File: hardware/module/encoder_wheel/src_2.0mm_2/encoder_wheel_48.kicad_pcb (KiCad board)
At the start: 2 copper layers, 74 x 74 mm, 2 parts

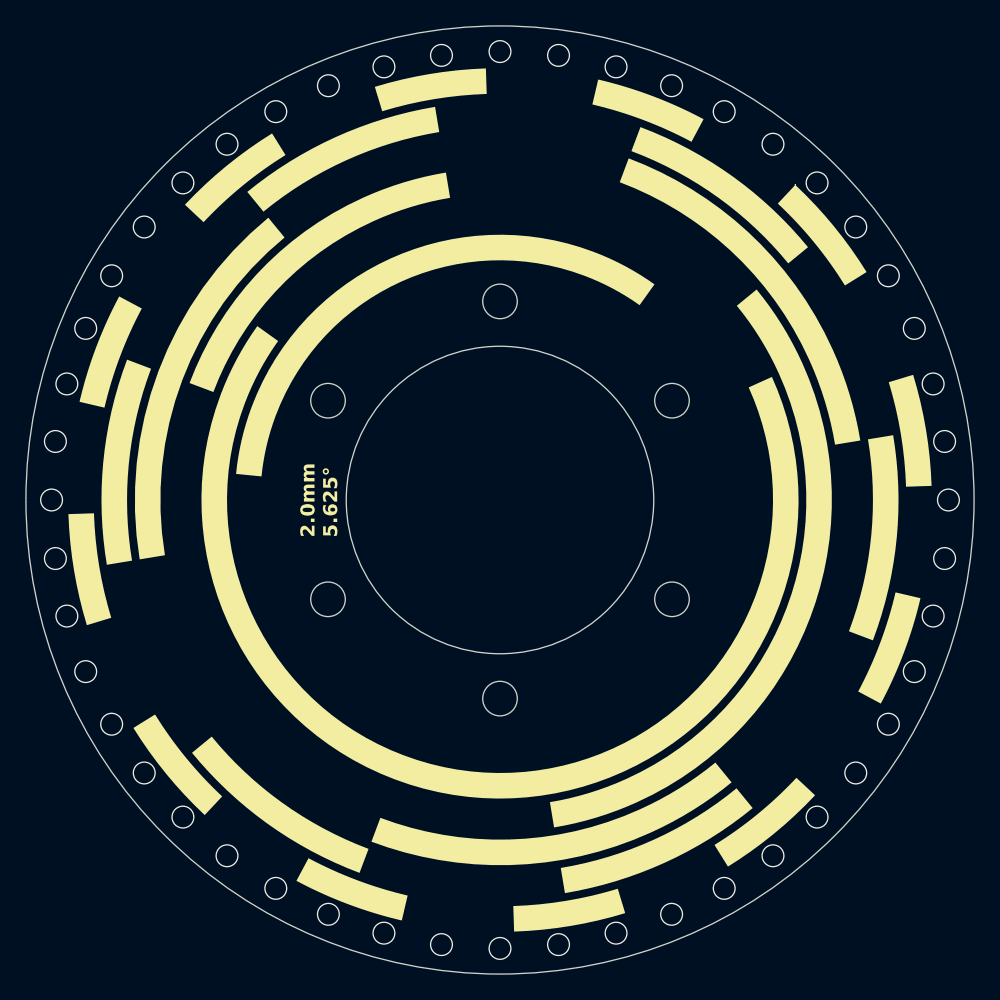
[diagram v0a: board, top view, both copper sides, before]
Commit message: encoder changes
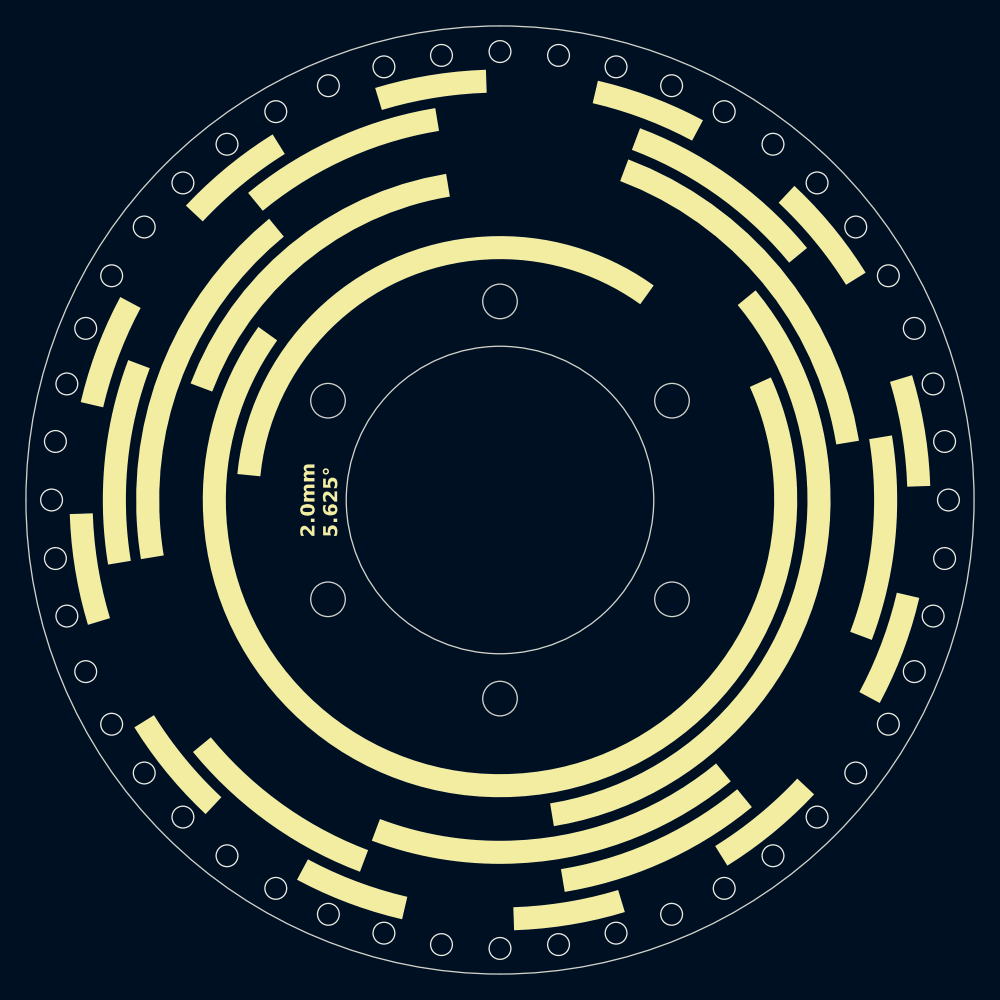
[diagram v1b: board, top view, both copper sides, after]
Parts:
- renumbered REF** to ENC1, REF** to ENC2
